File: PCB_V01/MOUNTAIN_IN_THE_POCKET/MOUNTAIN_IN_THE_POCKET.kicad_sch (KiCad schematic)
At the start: 9 parts, among them U1 AS1115-BSST

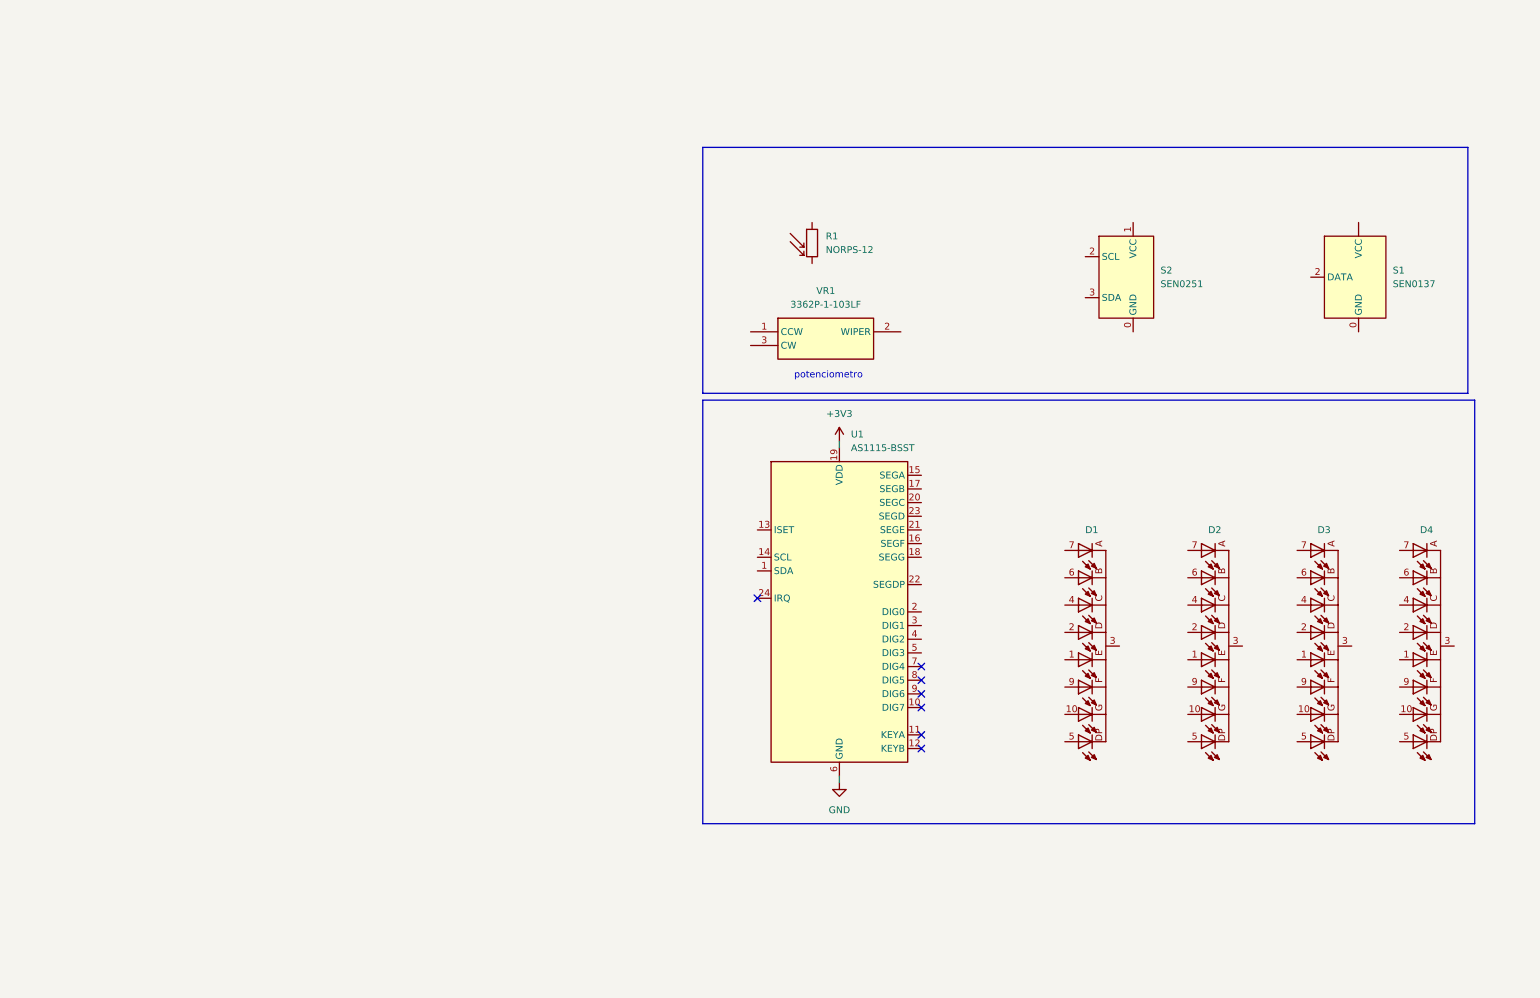
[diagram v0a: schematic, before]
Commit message: SCH en proceso
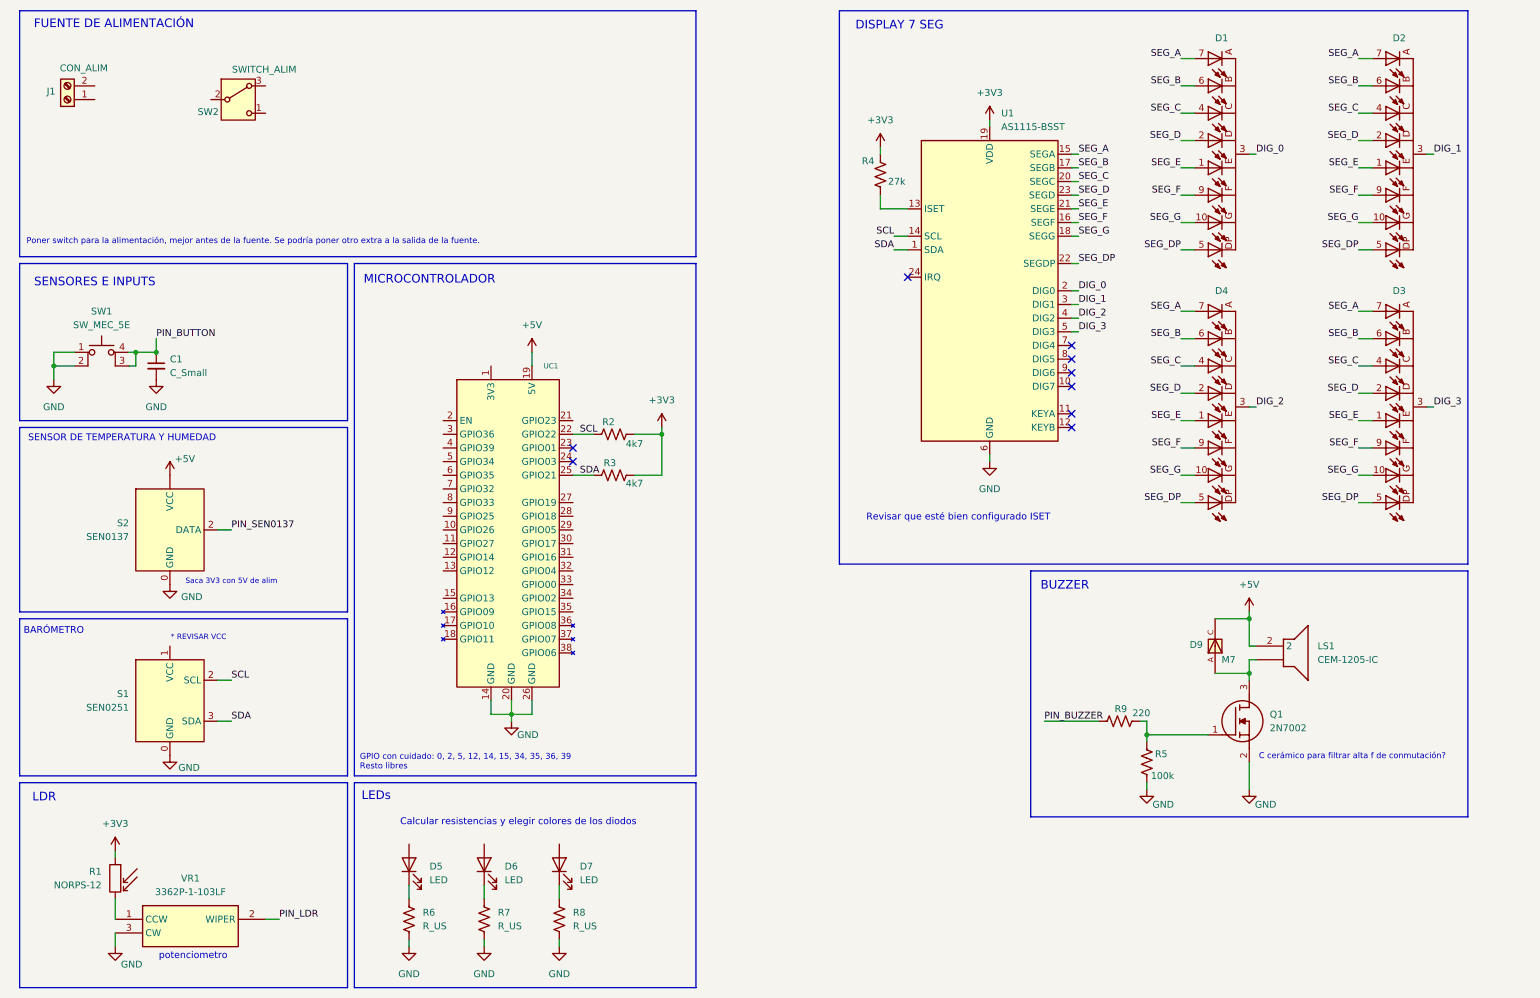
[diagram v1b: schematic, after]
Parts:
- removed S1: SEN0137, symbol COMPONENTES_SCH:SEN0137
- removed S2: SEN0251, symbol COMPONENTES_SCH:SEN0251
- added C1: C_Small, symbol Device:C_Small
- added D5, D6, D7: LED, symbol Device:LED
- added D9: M7, M7:DIOM505270X240, symbol M7:M7
- added J1: CON_ALIM, symbol Connector:Screw_Terminal_01x02
- added LS1: CEM-1205-IC, CEM1205IC, symbol CEM-1205-IC:CEM-1205-IC
- added Q1: 2N7002, SOT96P240X120-3N, symbol 2N7002:2N7002
- added R2, R3: 4k7, symbol Device:R_US
- added R4: 27k, symbol Device:R_US
- added R5: 100k, symbol Device:R_US
- added R6, R7, R8: R_US, symbol Device:R_US
- added R9: 220, symbol Device:R_US
- added S1: SEN0251, symbol COMPONENTES_SCH:SEN0251
- added S2: SEN0137, symbol COMPONENTES_SCH:SEN0137
- added SW1: SW_MEC_5E, symbol Switch:SW_MEC_5E
- added SW2: SWITCH_ALIM, Button_Switch_SMD:Nidec_Copal_CAS-120A, symbol Switch:SW_Nidec_CAS-120A1
- added UC1: (no value), ESP32_TOOLS_DIEGO:ESP32_WROOM32_SHIELD_V01, symbol ESP32_TOOLS_DIEGO:ESP32_WROOM32_SHIELD_V01
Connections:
- net +3V3: now also R1.1, R2.2, R3.1, R4.1
- net GND: now also VR1.3 (CW), C1.2, Q1.2 (S), R5.1, R6.1, R7.1, R8.1, S1.0 (GND), S2.0 (GND), SW1.1, SW1.2, UC1.14 (GND), UC1.20 (GND), UC1.26 (GND)
- net SEG_E: now reaches D3.1 (E)
- net SEG_E: now also D1.1 (E), D2.1 (E), D4.1 (E), U1.21 (SEGE)
- net SEG_G: now reaches D3.10 (G)
- net SEG_G: now also D1.10 (G), D2.10 (G), D4.10 (G), U1.18 (SEGG)
- net SEG_D: now reaches D3.2 (D)
- net SEG_D: now also D1.2 (D), D2.2 (D), D4.2 (D), U1.23 (SEGD)
- net DIG_3: now reaches D3.3, D3.8
- net DIG_3: now also U1.5 (DIG3)
- net SEG_C: now reaches D3.4 (C)
- net SEG_C: now also D1.4 (C), D2.4 (C), D4.4 (C), U1.20 (SEGC)
- net SEG_DP: now reaches D3.5 (DP)
- net SEG_DP: now also D1.5 (DP), D2.5 (DP), D4.5 (DP), U1.22 (SEGDP)
- net SEG_B: now reaches D3.6 (B)
- net SEG_B: now also D1.6 (B), D2.6 (B), D4.6 (B), U1.17 (SEGB)
- net SEG_A: now reaches D3.7 (A)
- net SEG_A: now also D1.7 (A), D2.7 (A), D4.7 (A), U1.15 (SEGA)
- net SEG_F: now reaches D3.9 (F)
- net SEG_F: now also D1.9 (F), D2.9 (F), D4.9 (F), U1.16 (SEGF)
- net DIG_1: now reaches D2.3, D2.8
- net DIG_1: now also U1.3 (DIG1)
- net DIG_2: now reaches D4.3, D4.8
- net DIG_2: now also U1.4 (DIG2)
- net at VR1.1 (CCW): now also R1.2
- net PIN_LDR: now reaches VR1.2 (WIPER)
- net DIG_0: now reaches D1.3, D1.8
- net DIG_0: now also U1.2 (DIG0)
- net SDA: now reaches U1.1 (SDA)
- net SDA: now also R3.2, S1.3 (SDA), UC1.25 (GPIO21)
- net at U1.13 (ISET): now also R4.2
- net SCL: now reaches U1.14 (SCL)
- net SCL: now also R2.1, S1.2 (SCL), UC1.22 (GPIO22)
- new net: D9.A, LS1., Q1.3 (D)
- new net: D5.1 (K), R6.2
- new net: D7.1 (K), R8.2
- new net: Q1.1 (G), R5.2, R9.1
- new net: D6.1 (K), R7.2
- new net +5V: D9.C, LS1.2, S2. (VCC), UC1.19 (5V)
- new net PIN_BUTTON: C1.1, SW1.3 (K), SW1.4 (A)
- new net PIN_BUZZER: R9.2
- new net PIN_SEN0137: S2.2 (DATA)
- no-connect marks 7 -> 9
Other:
- note added: "* REVISAR VCC"
- note added: "BARÓMETRO"
- note added: "BUZZER"
- note added: "C cerámico para filtrar alta f de conmutación?"
- note added: "Calcular resistencias y elegir colores de los diodos"
- note added: "DISPLAY 7 SEG"
- note added: "FUENTE DE ALIMENTACIÓN"
- note added: "GPIO con cuidado: 0, 2, 5, 12, 14, 15, 34, 35, 36, 39 Resto libres"
- note added: "LDR"
- note added: "LEDs"
- note added: "MICROCONTROLADOR"
- note added: "Poner switch para la alimentación, mejor antes de la fuente. Se podría poner otro extra a la salida de la fuente."
- note added: "Revisar que esté bien configurado ISET"
- note added: "SENSOR DE TEMPERATURA Y HUMEDAD"
- note added: "SENSORES E INPUTS"
- note added: "Saca 3V3 con 5V de alim"
- moved on the sheet: R1, U1
